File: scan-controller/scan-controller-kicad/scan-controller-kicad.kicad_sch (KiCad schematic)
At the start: 36 parts, among them CN1 24V in, J1 FTDI, J5 ICSP, J6 Raspi UART, J7 Raspi GPIO, Q2 IRLML2502, Q3 IRLML6402, SW3 Reset, U5 ATmega328P, Y1 8MHz

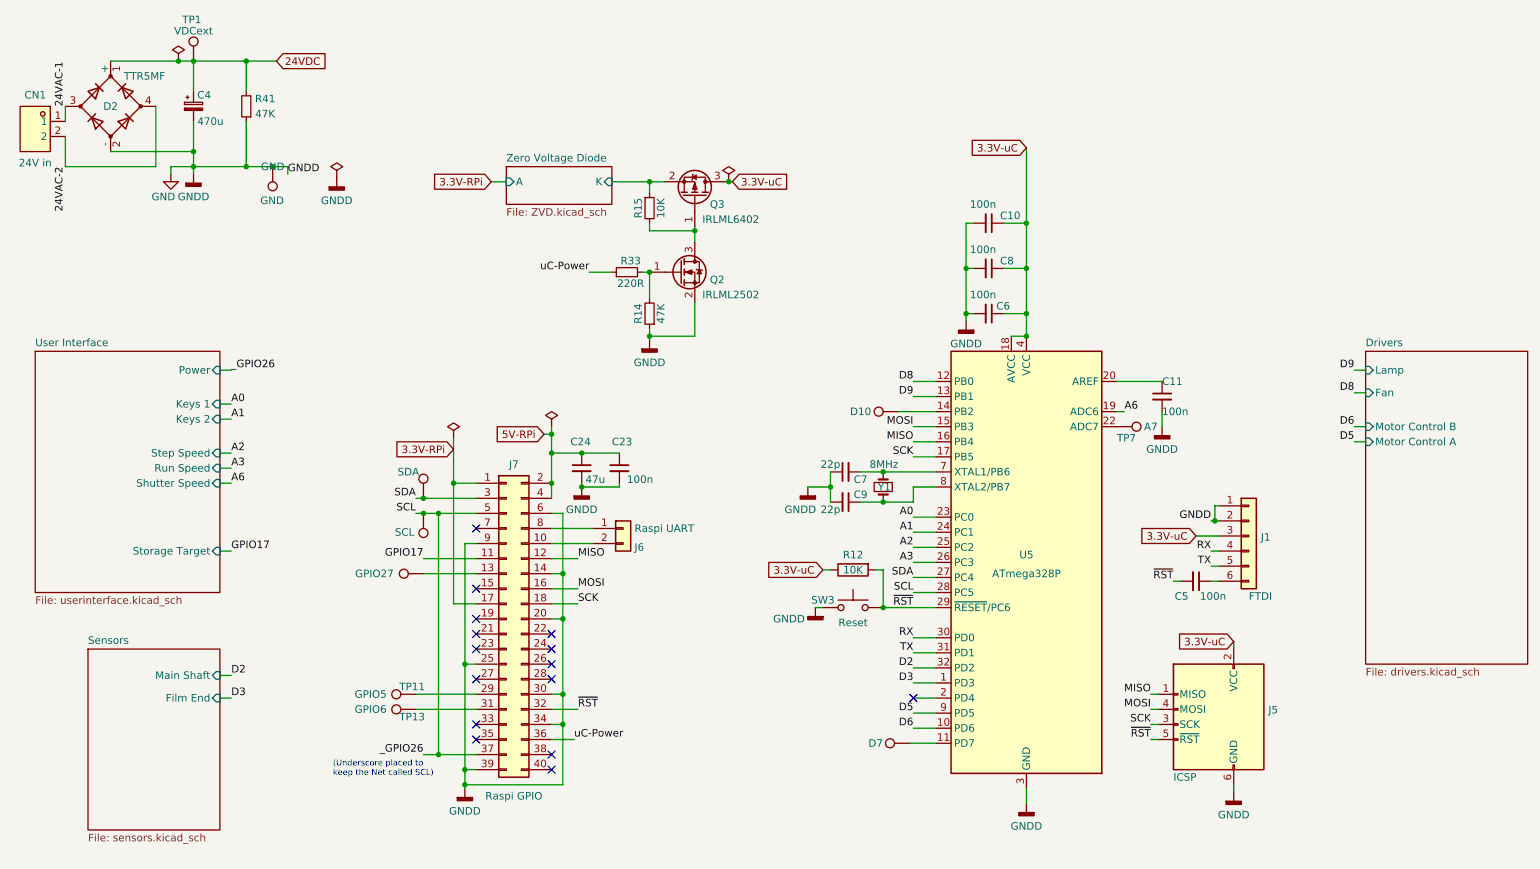
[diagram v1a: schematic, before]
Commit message: Raspi Power LED
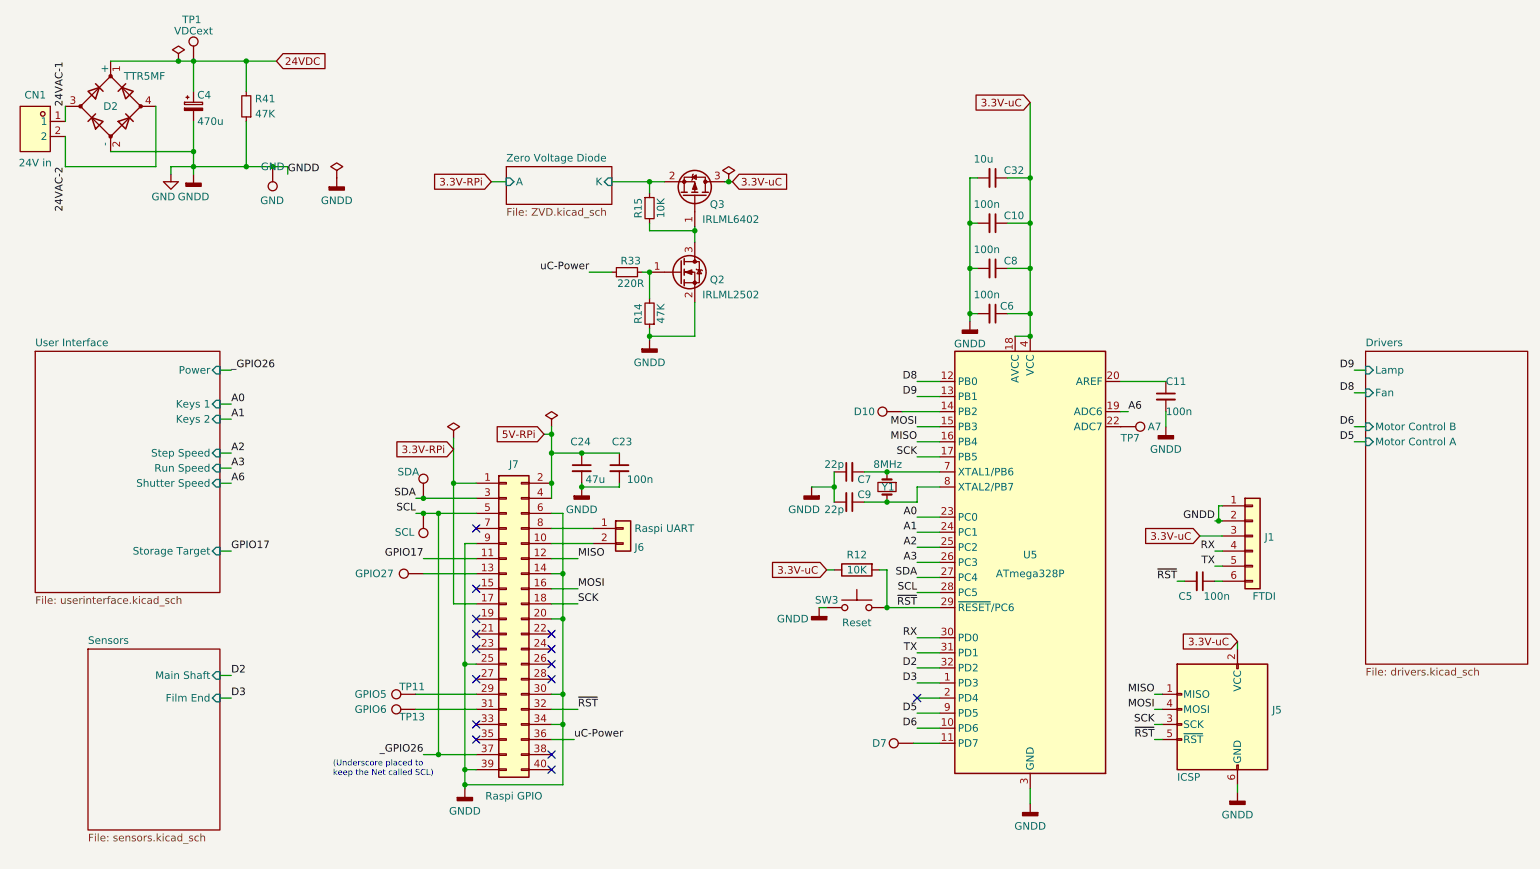
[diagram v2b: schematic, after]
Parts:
- added C32: 10u, Capacitor_SMD:C_0805_2012Metric, symbol Device:C_Small
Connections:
- net 3.3V-uC: now also C32.1
- net GND: now also C32.2
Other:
- moved on the sheet: C10, C11, C5, C6, C7, C8, C9, J1, J5, R12, SW3, TP7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

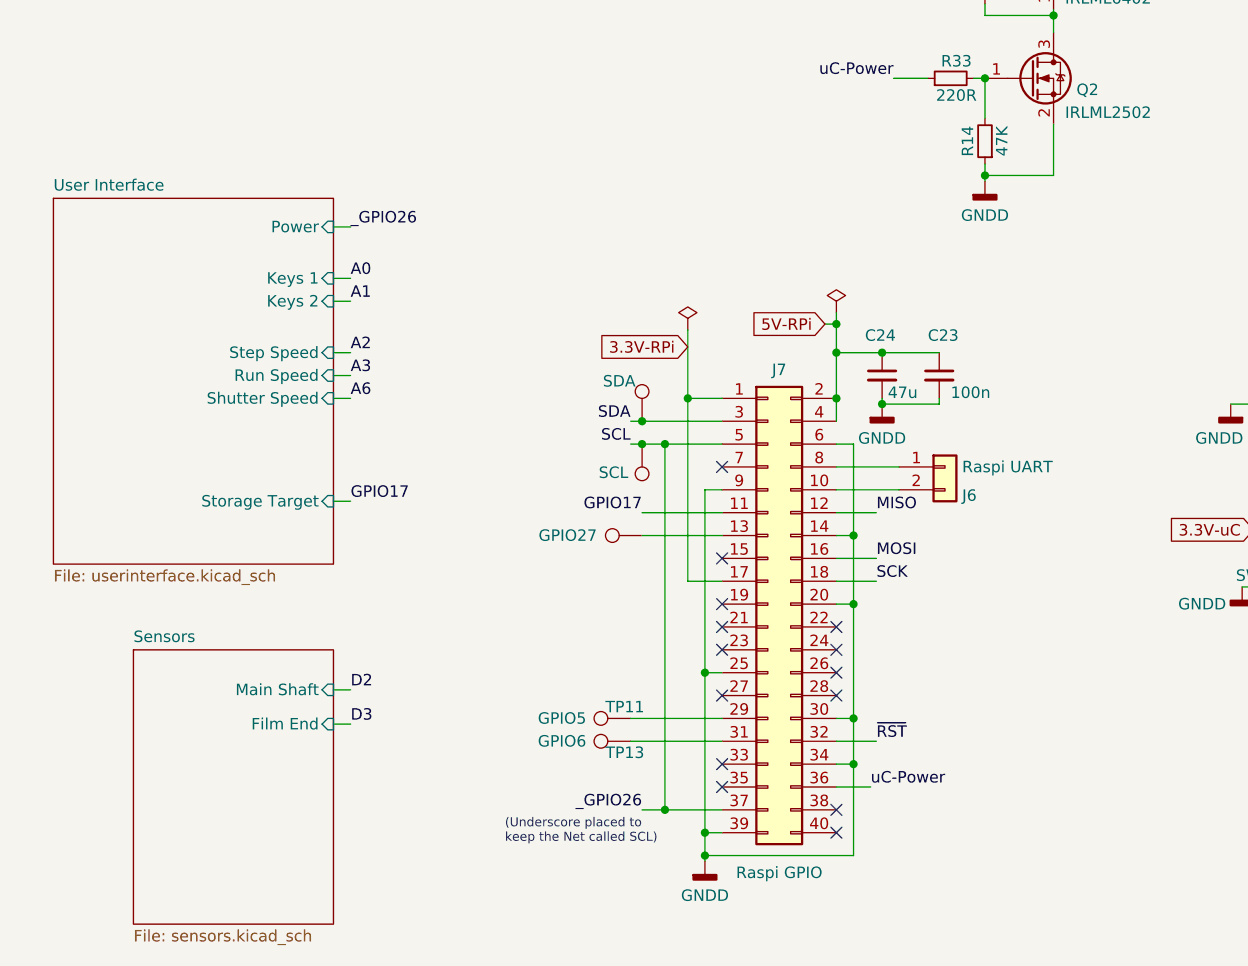
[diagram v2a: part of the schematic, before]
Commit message: Rename Target Switch to Resolution, add actual Target Switch
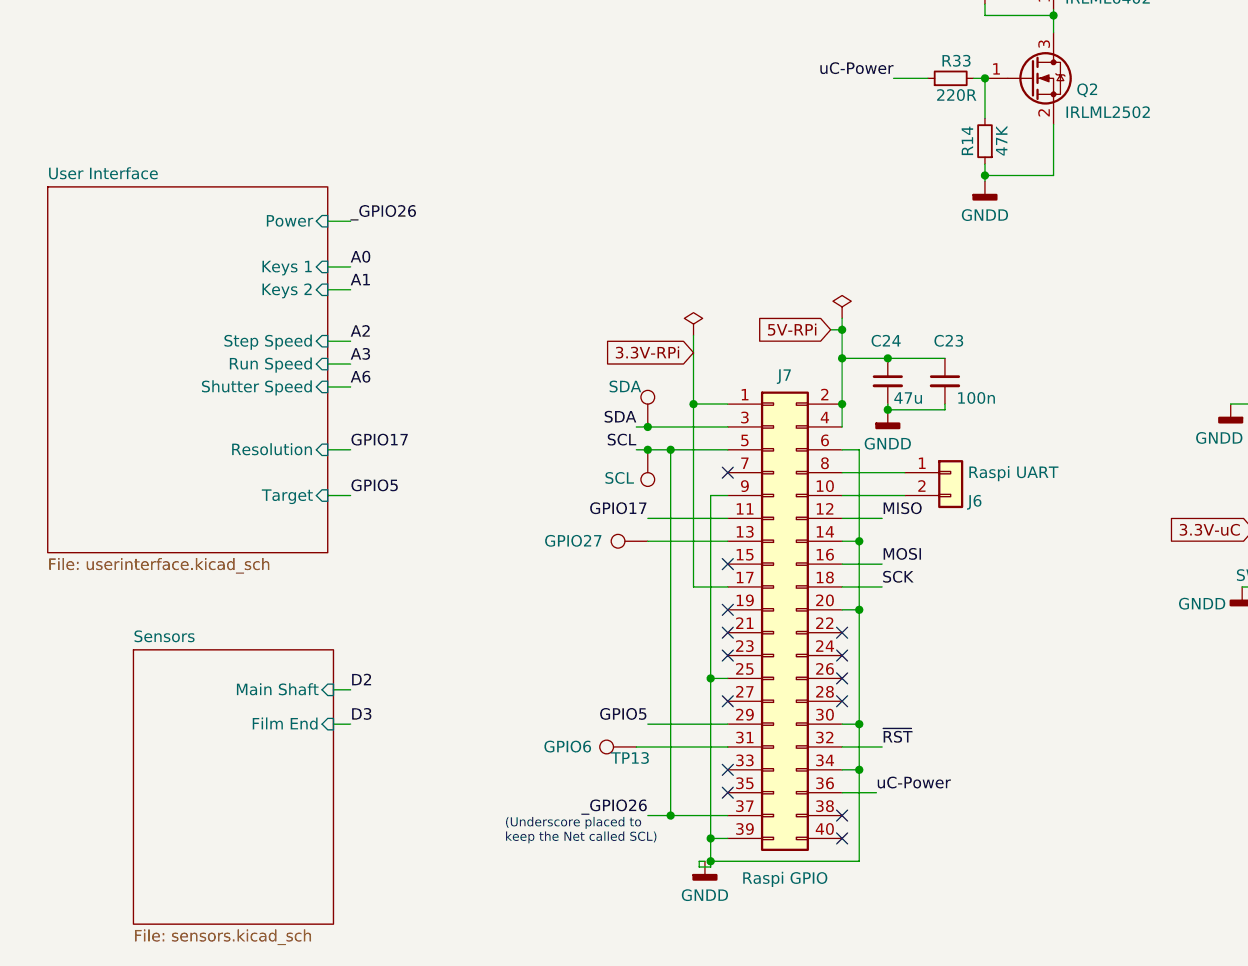
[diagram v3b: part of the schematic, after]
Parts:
- removed TP11: GPIO5, Peacemans_Footprints:TestPoint_THTPad_1.5x1.5mm_Drill0.7mm_named, symbol Peacemans_Teile:TestPoint_named
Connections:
- net GPIO5: now reaches J7.29 (Pin_29)
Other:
- sheet User Interface ports: added Resolution, Target; removed Storage Target
- moved on the sheet: C23, C24, J6, J7, TP13

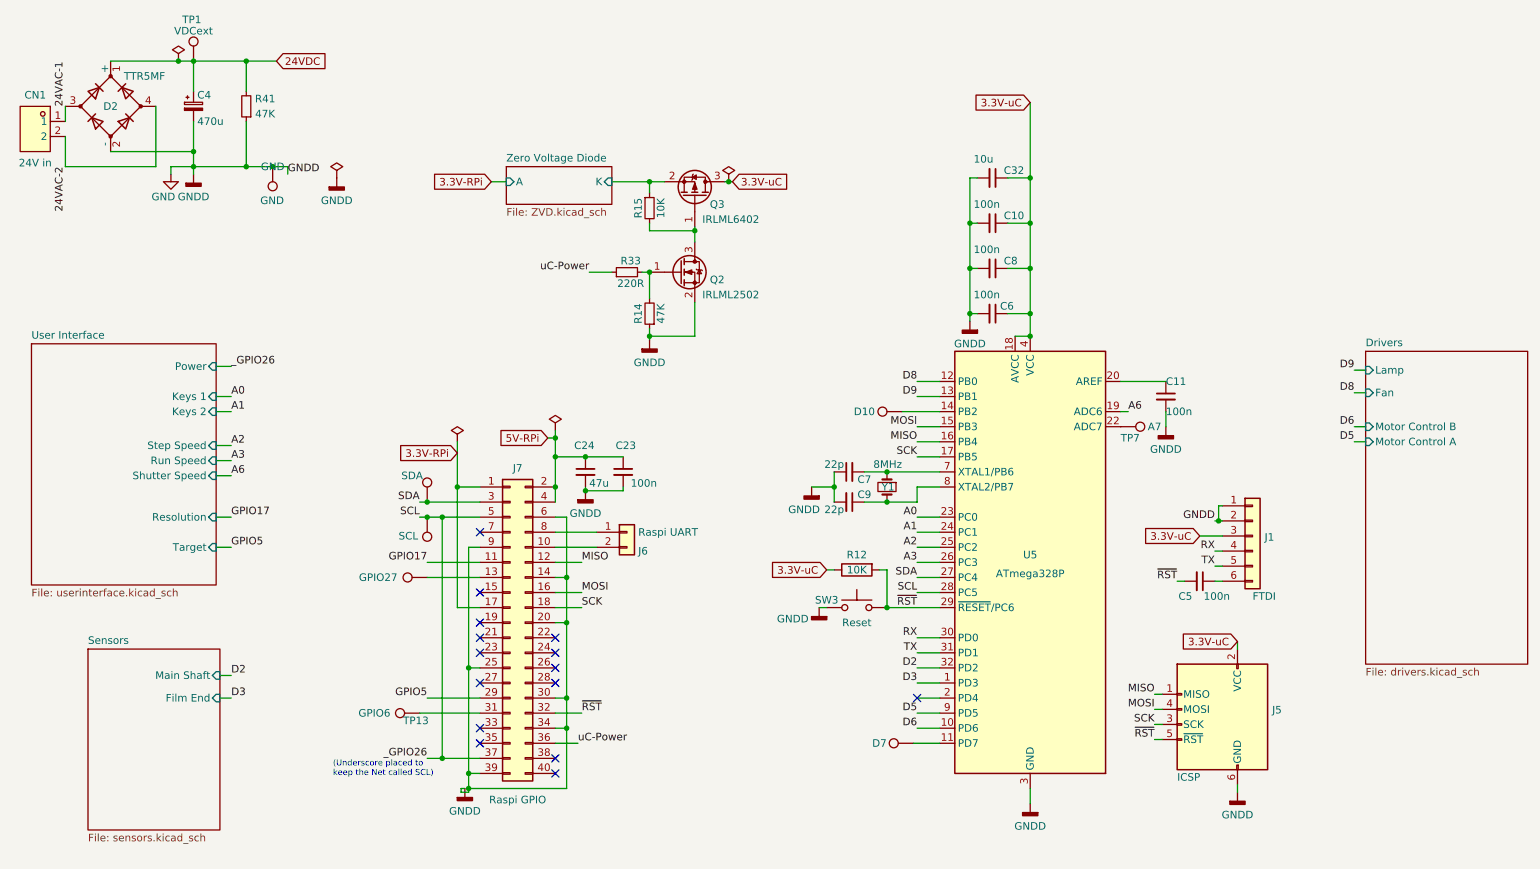
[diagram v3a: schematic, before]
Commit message: GND TP @ GPIO
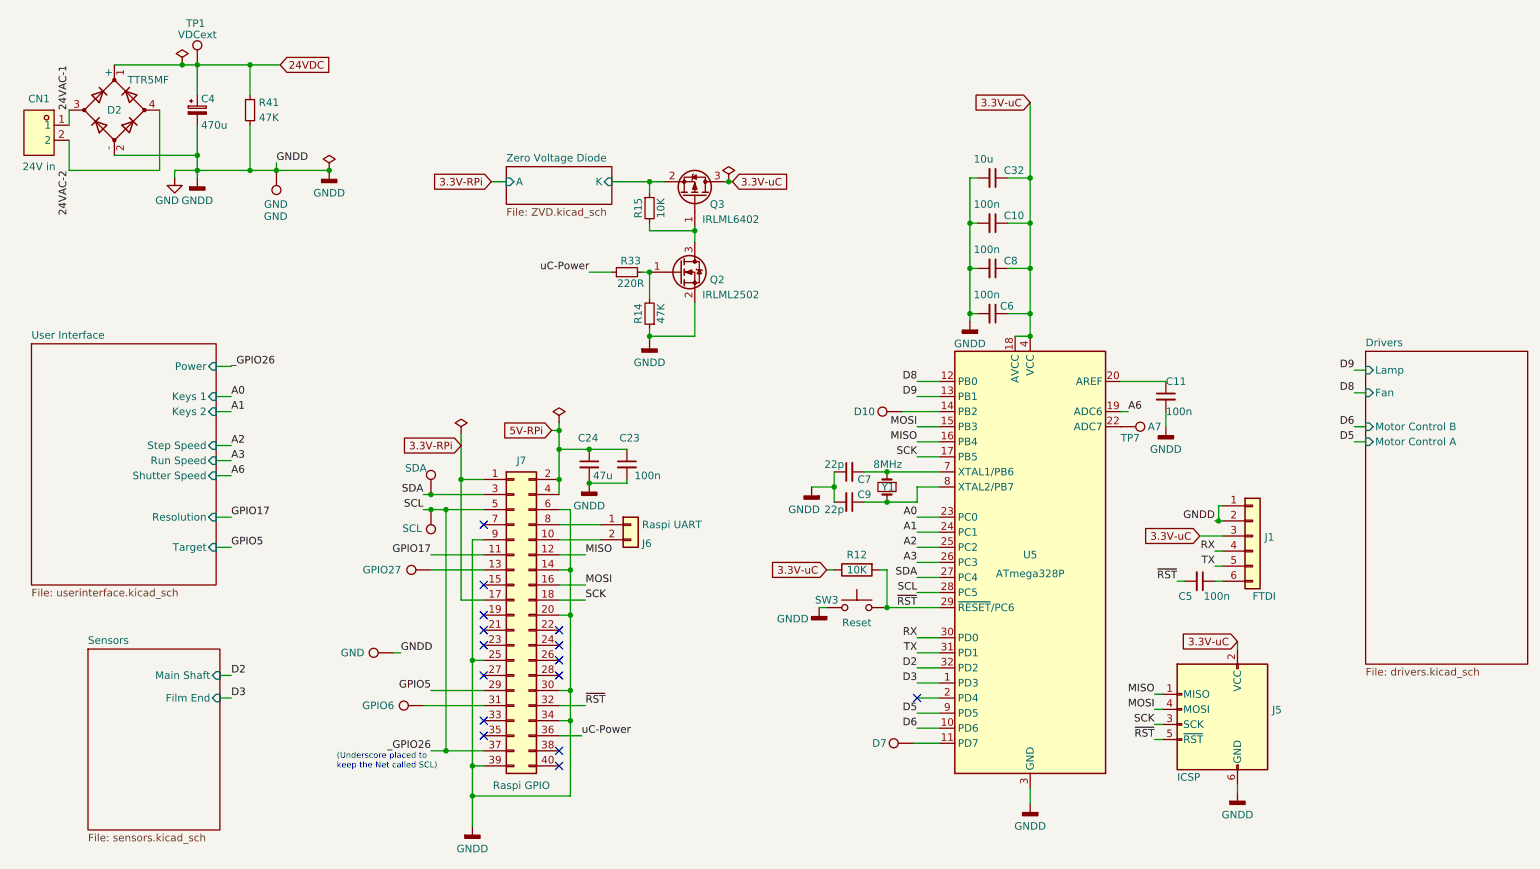
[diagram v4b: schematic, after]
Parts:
- added TP11: GND, Peacemans_Footprints:TestPoint_THTPad_1.5x1.5mm_Drill0.7mm_named, symbol Peacemans_Teile:TestPoint_named
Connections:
- net GND: now also TP11.1
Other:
- moved on the sheet: C23, C24, C4, CN1, D2, J6, J7, R41, TP1

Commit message: reassigned customfootprints to now gobal library
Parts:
- TP1, TP11, TP12, TP13, TP2, TP4, TP5, TP6, TP7, TP8: footprint Peacemans_Footprints:TestPoint_THTPad_1.5x1.5mm_Drill0.7mm_named -> Peacemans_Teile:TestPoint_THTPad_1.5x1.5mm_Drill0.7mm_named
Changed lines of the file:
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@@
 			)
 		)
-		(property "Footprint" "Peacemans_Footprints:TestPoint_THTPad_1.5x1.5mm_Drill0.7mm_named"
+		(property "Footprint" "Peacemans_Teile:TestPoint_THTPad_1.5x1.5mm_Drill0.7mm_named"
 			(at 53.975 24.13 0)
 			(effects
@@
 			)
 		)
-		(property "Footprint" "Peacemans_Footprints:TestPoint_THTPad_1.5x1.5mm_Drill0.7mm_named"
+		(property "Footprint" "Peacemans_Teile:TestPoint_THTPad_1.5x1.5mm_Drill0.7mm_named"
 			(at 86.995 127 0)
 			(effects
@@
 			)
 		)
-		(property "Footprint" "Peacemans_Footprints:TestPoint_THTPad_1.5x1.5mm_Drill0.7mm_named"
+		(property "Footprint" "Peacemans_Teile:TestPoint_THTPad_1.5x1.5mm_Drill0.7mm_named"
 			(at 83.185 99.06 0)
 			(effects
@@
 			)
 		)
-		(property "Footprint" "Peacemans_Footprints:TestPoint_THTPad_1.5x1.5mm_Drill0.7mm_named"
+		(property "Footprint" "Peacemans_Teile:TestPoint_THTPad_1.5x1.5mm_Drill0.7mm_named"
 			(at 81.915 118.11 0)
 			(effects
@@
 			)
 		)
-		(property "Footprint" "Peacemans_Footprints:TestPoint_THTPad_1.5x1.5mm_Drill0.7mm_named"
+		(property "Footprint" "Peacemans_Teile:TestPoint_THTPad_1.5x1.5mm_Drill0.7mm_named"
 			(at 204.47 80.01 0)
 			(effects
@@
 			)
 		)
-		(property "Footprint" "Peacemans_Footprints:TestPoint_THTPad_1.5x1.5mm_Drill0.7mm_named"
+		(property "Footprint" "Peacemans_Teile:TestPoint_THTPad_1.5x1.5mm_Drill0.7mm_named"
 			(at 88.265 104.14 0)
 			(effects
@@
 			)
 		)
-		(property "Footprint" "Peacemans_Footprints:TestPoint_THTPad_1.5x1.5mm_Drill0.7mm_named"
+		(property "Footprint" "Peacemans_Teile:TestPoint_THTPad_1.5x1.5mm_Drill0.7mm_named"
 			(at 169.545 143.51 0)
 			(effects
@@
 			)
 		)
-		(property "Footprint" "Peacemans_Footprints:TestPoint_THTPad_1.5x1.5mm_Drill0.7mm_named"
+		(property "Footprint" "Peacemans_Teile:TestPoint_THTPad_1.5x1.5mm_Drill0.7mm_named"
 			(at 167.64 87.63 0)
 			(effects
@@
 			)
 		)
-		(property "Footprint" "Peacemans_Footprints:TestPoint_THTPad_1.5x1.5mm_Drill0.7mm_named"
+		(property "Footprint" "Peacemans_Teile:TestPoint_THTPad_1.5x1.5mm_Drill0.7mm_named"
 			(at 57.15 41.91 0)
 			(effects
@@
 			)
 		)
-		(property "Footprint" "Peacemans_Footprints:TestPoint_THTPad_1.5x1.5mm_Drill0.7mm_named"
+		(property "Footprint" "Peacemans_Teile:TestPoint_THTPad_1.5x1.5mm_Drill0.7mm_named"
 			(at 93.345 96.52 0)
 			(effects
